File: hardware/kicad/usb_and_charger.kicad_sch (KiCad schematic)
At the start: 15 parts, among them J2 USB_C_Receptacle_USB2.0, U1 MCP73831-2-OT, U2 USBLC6-2SC6

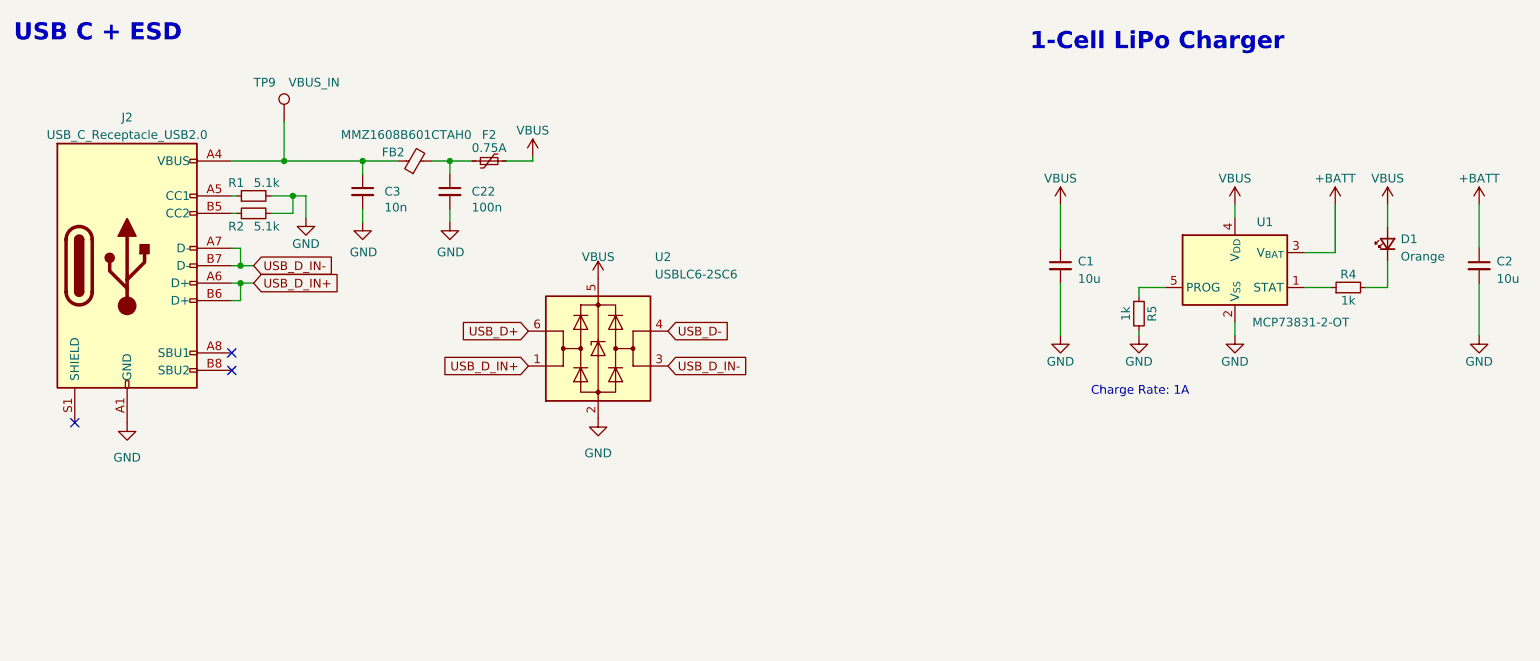
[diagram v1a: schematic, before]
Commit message: wip: revision 2
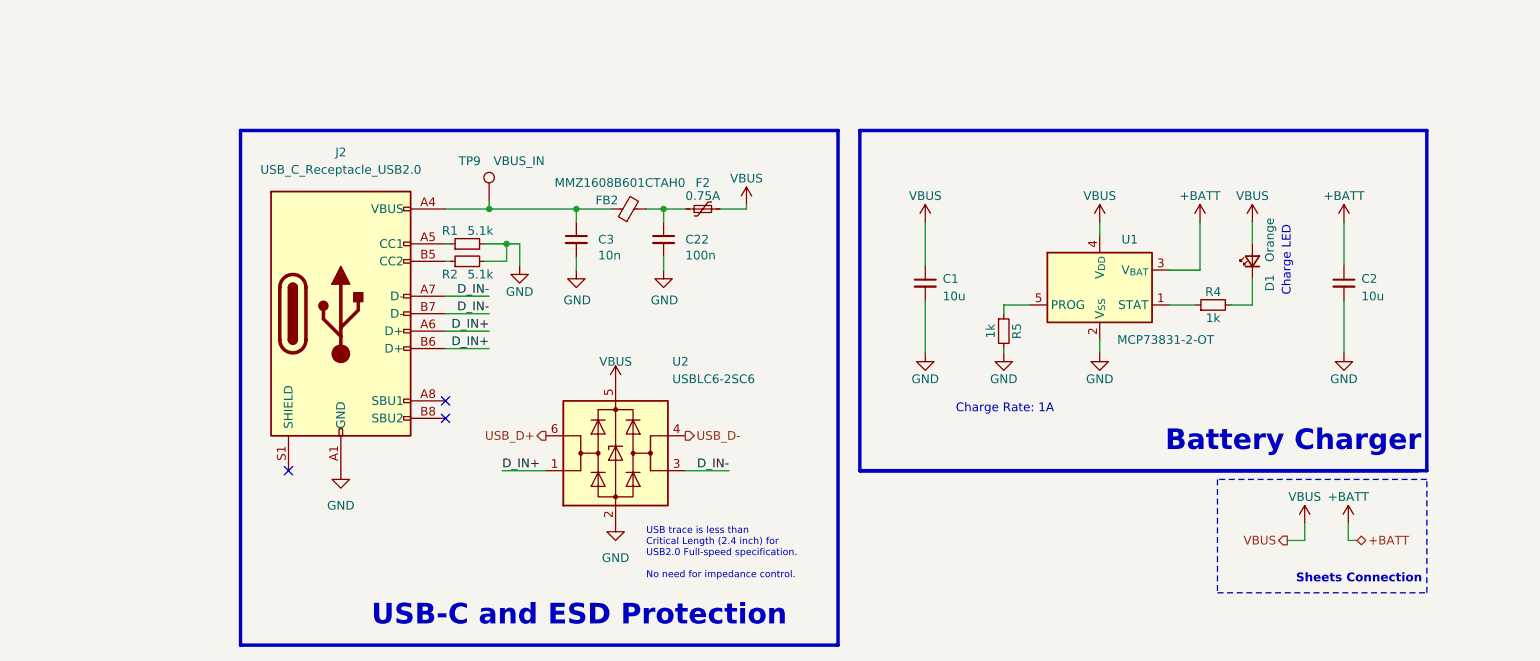
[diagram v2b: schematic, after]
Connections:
- net USB_D_IN+ renamed D_IN+
- net USB_D_IN- renamed D_IN-
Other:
- note added: "Battery Charger"
- note added: "Charge LED"
- note added: "Sheets Connection"
- note added: "USB trace is less than Critical Length (2.4 inch) for USB2.0 Full-speed specification. No need for impedance control."
- note added: "USB-C and ESD Protection"
- note removed: "1-Cell LiPo Charger"
- note removed: "USB C + ESD"
- moved on the sheet: C1, C2, C22, C3, D1, F2, FB2, J2, R1, R2, R4, R5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
